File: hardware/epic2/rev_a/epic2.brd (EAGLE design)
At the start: 18 x 18 mm, 33 parts, among them J1 EPIC2-HEADER2, U1 RV-4162-C7, U2 FM25LBTDFN-8, U3 CC2538, X1 EPSON-FA-128, X3 ABS05-32.768KHZ-T

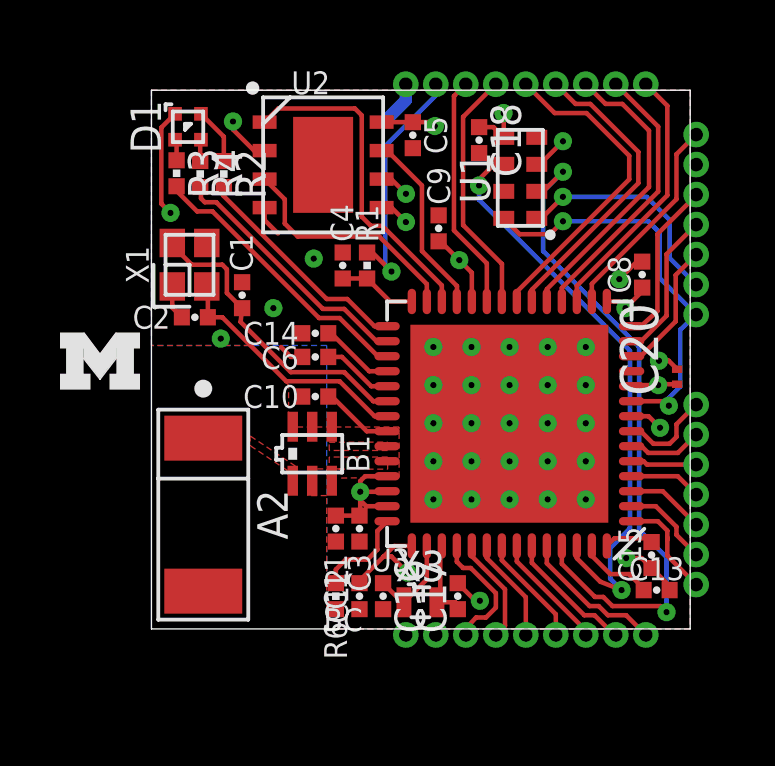
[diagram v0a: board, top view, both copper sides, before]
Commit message: no airwaires
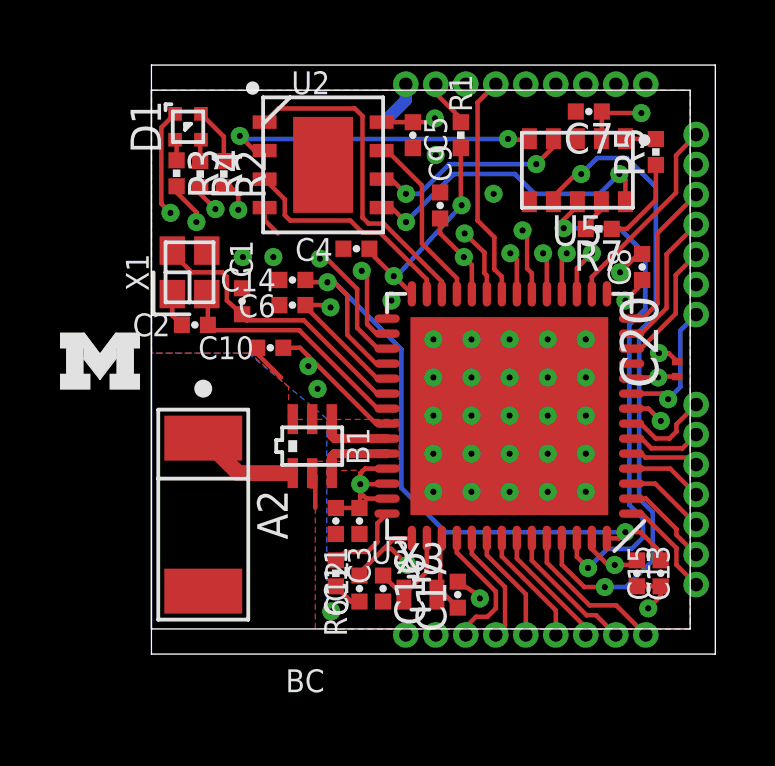
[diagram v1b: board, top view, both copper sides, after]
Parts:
- removed C18: 10nF, passives:0402_CAP
- removed U1: RV-4162-C7, chips:MICRO-CRYSTAL-C7
- added C7: 10nF, passives:0402_CAP
- added R5, R7: 10k, passives:0402_RES
- added U5: RV-3049-C3, chips:MICRO-CRYSTAL-C3
- moved R1 5.35 mm to (10.3, 16.5)
- moved C10 2.21 mm to (3.96, 9.37)
- moved C14 1.93 mm to (4.70, 11.6)
- moved C6 1.89 mm to (4.70, 10.8)
- moved C13 0.87 mm to (16.2, 1.85), turned to 270 degrees
- moved C9 0.76 mm to (9.62, 14.1)
- moved R6 0.76 mm to (6.15, 1.85)
- moved C4 0.72 mm to (6.83, 12.7), turned to 180 degrees
- moved C15 0.68 mm to (17.0, 1.85)
- moved B1 0.25 mm to (5.36, 6.09)
- moved C11 0.25 mm to (6.15, 3.60)
- moved C12 0.25 mm to (6.93, 1.35)
- moved C16 0.25 mm to (7.72, 1.35)
- moved C3 0.25 mm to (6.93, 3.60)
- moved X3 0.25 mm to (8.97, 1.14)
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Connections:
- removed net RTC_CLKOUT: U1.2, U3.53
- new net !RTC_CS: U3.54, U5.8
- new net N$14: R7.2, U5.9
- new net N$16: R5.2, U5.1
- net !RTC_INT: now also U3.53, U5.7; no longer U1.6, U3.54
- net GND: now also C7.2, R5.1, R7.1, U5.6; no longer C18.2, U1.3
- net I2C_SCL: no longer U1.8
- net I2C_SDA: no longer U1.1
- net SPI_MISO: now also U5.5
- net SPI_MOSI: now also U5.10
- net SPI_SCK: now also U5.4
- net VCC: now also C7.1, U5.2; no longer C18.1, U1.5
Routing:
- net RTC_CLKOUT: track 22.6 -> 0.00 mm, vias 2 -> 0
- net N$15: track 4.18 -> 23.2 mm, vias 0 -> 2
- net !RTC_CS: track 0.00 -> 17.4 mm, vias 0 -> 2
- net SPI_MOSI: track 19.4 -> 29.0 mm, vias 1 -> 2
- net I2C_SCL: track 13.7 -> 4.50 mm, vias 2 -> 1
- net SPI_MISO: track 26.0 -> 34.5 mm, vias 1 -> 2
- net I2C_SDA: track 14.6 -> 6.87 mm, vias 2 -> 1
- net SPI_SCK: track 18.5 -> 26.0 mm, vias 1 -> 2
- net !RESET: track 8.10 -> 1.61 mm, vias 1 -> 0
- net VCC: track 29.6 -> 34.8 mm, vias 8 -> 11
- net N$1: track 2.62 -> 7.36 mm, vias 0 -> 2
- net GND: track 11.7 -> 15.9 mm, vias 33 -> 35
- net ANTENNA: track 0.00 -> 3.47 mm
- net ADC5: track 10.8 -> 8.31 mm, vias 0 -> 1
- net ADC4: track 10.1 -> 7.64 mm, vias 0 -> 1
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- removed copper zone on layer 1, net ANTENNA
- removed copper zone on layer 1, net RF_N
- removed copper zone on layer 1, net RF_P
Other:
- board size 18 x 18 mm -> 18.8 x 19.6 mm
